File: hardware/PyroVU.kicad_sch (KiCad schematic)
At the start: 48 parts, among them IC1 TM1637__SOP_, J1 Conn_01x05_Pin, J2 Screw_Terminal_01x02, J3 Screw_Terminal_01x02, J4 Screw_Terminal_01x02, U1 MAX31856, U2 MAX31865xAP, U3 SM420561N, U4 SM420561N, U5 SM420561N, U6 SM420561N, U7 SM420561N, U8 SM420561N

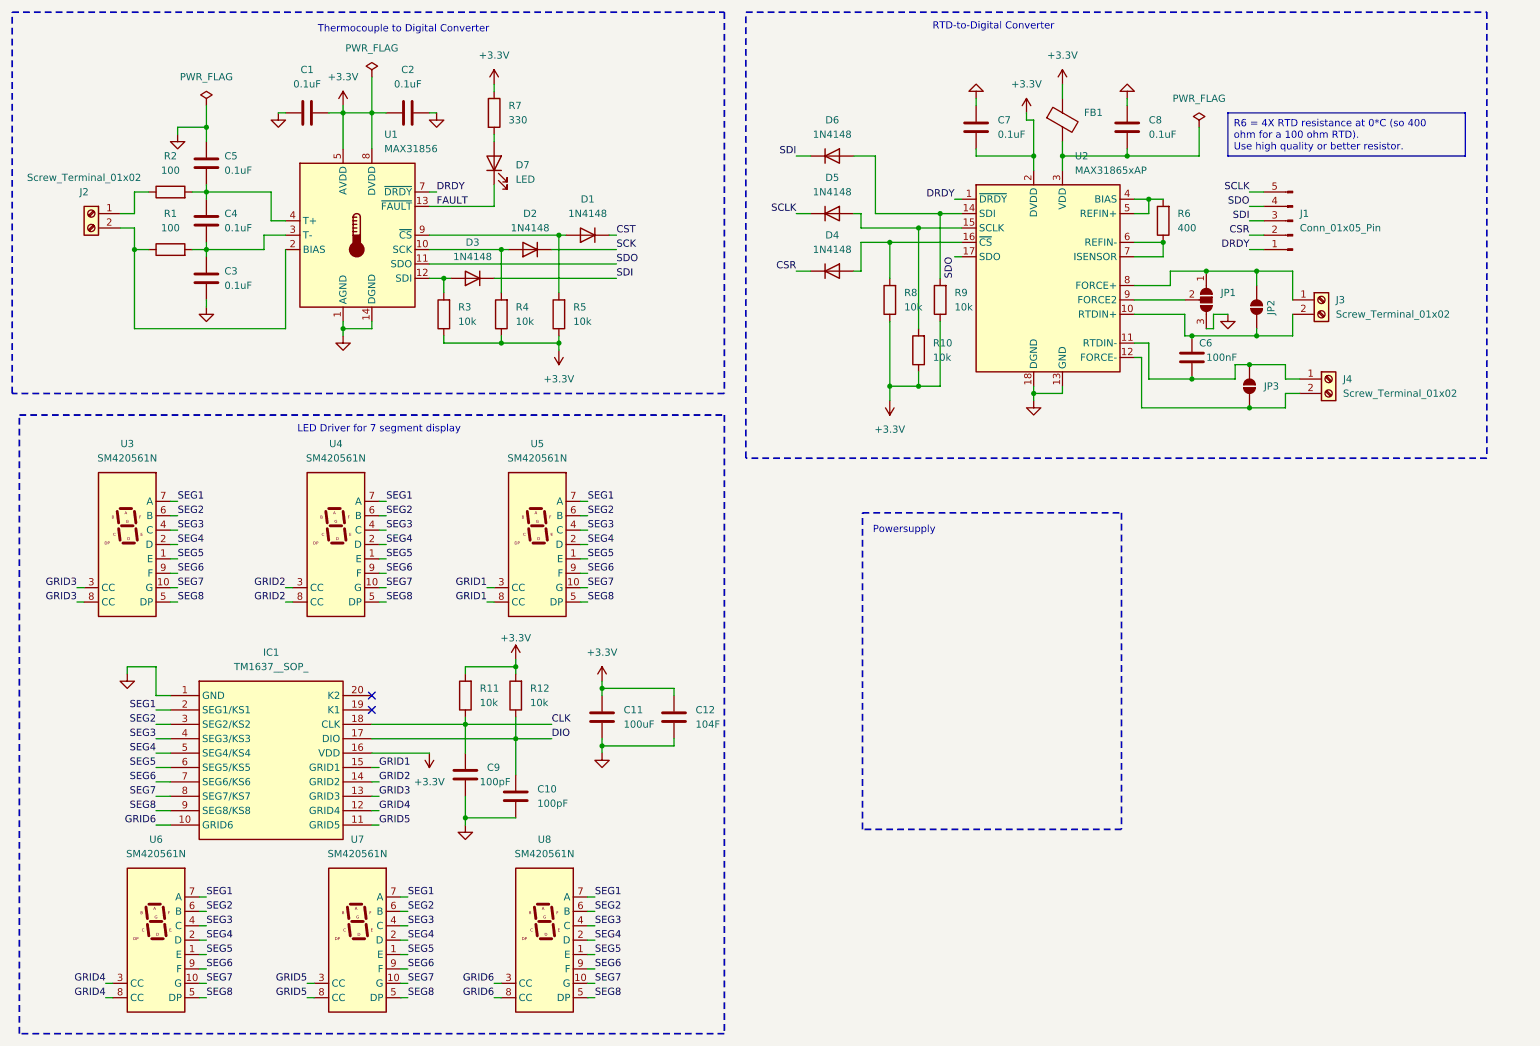
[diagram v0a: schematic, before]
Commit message: Changes in the Schematic
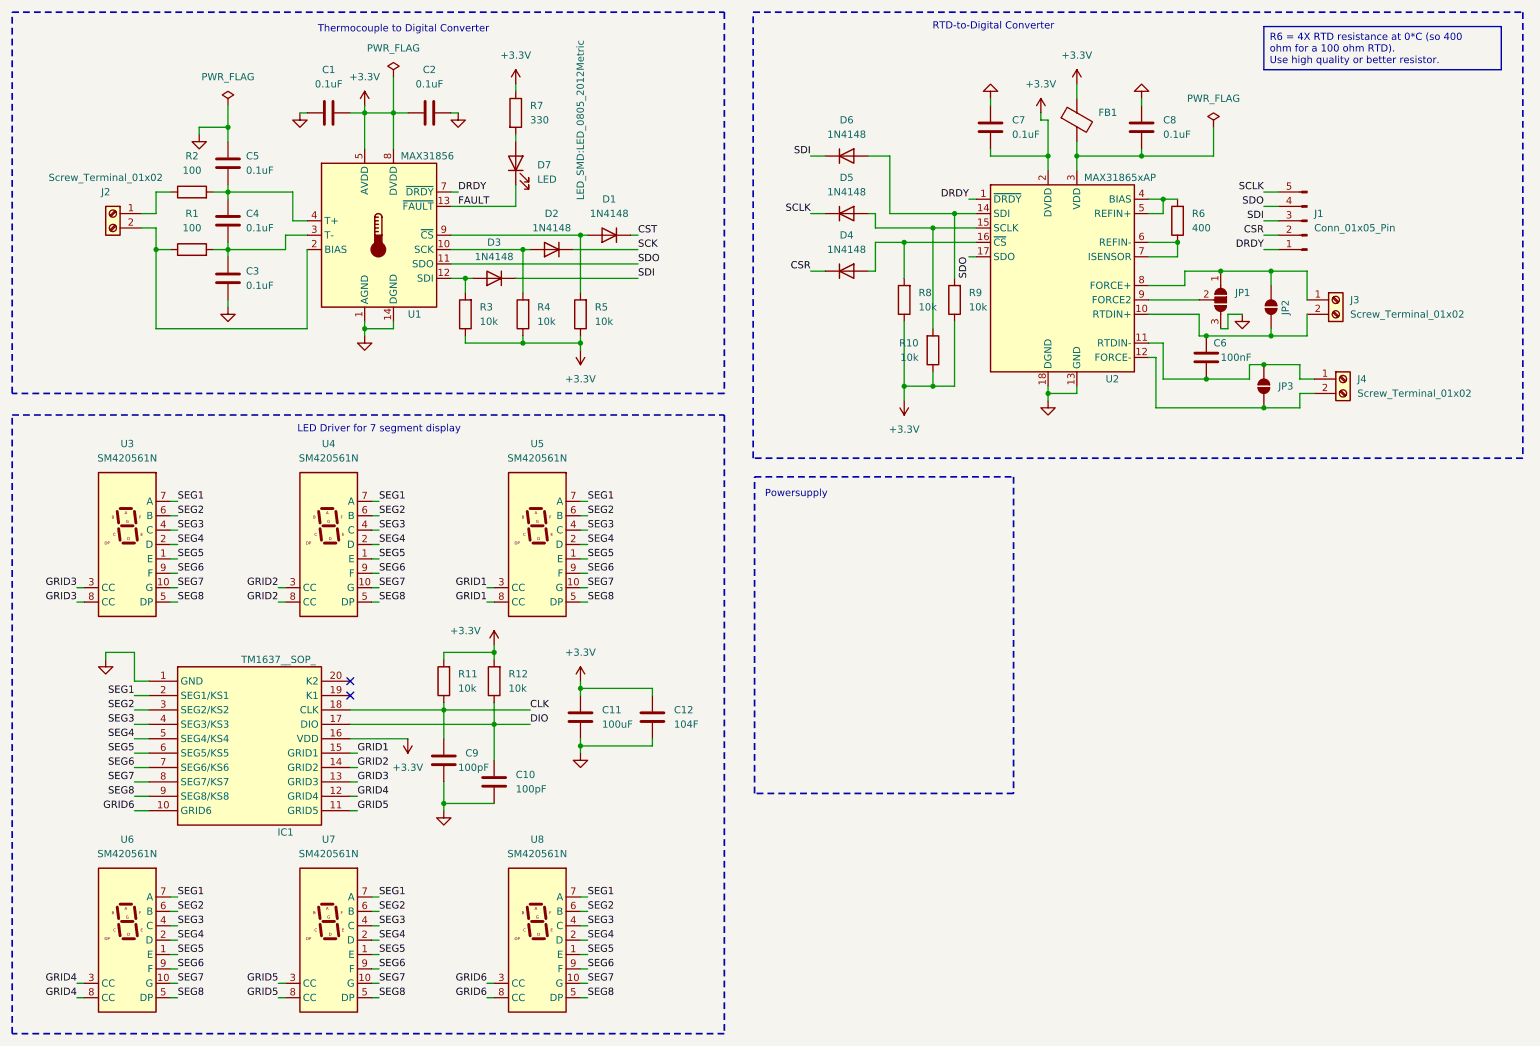
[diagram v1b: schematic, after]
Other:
- moved on the sheet: C1, C10, C11, C12, C2, C3, C4, C5, C6, C7, C8, C9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
